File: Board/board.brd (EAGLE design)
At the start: 68.6 x 53.3 mm, 19 parts, among them IC1 L293D

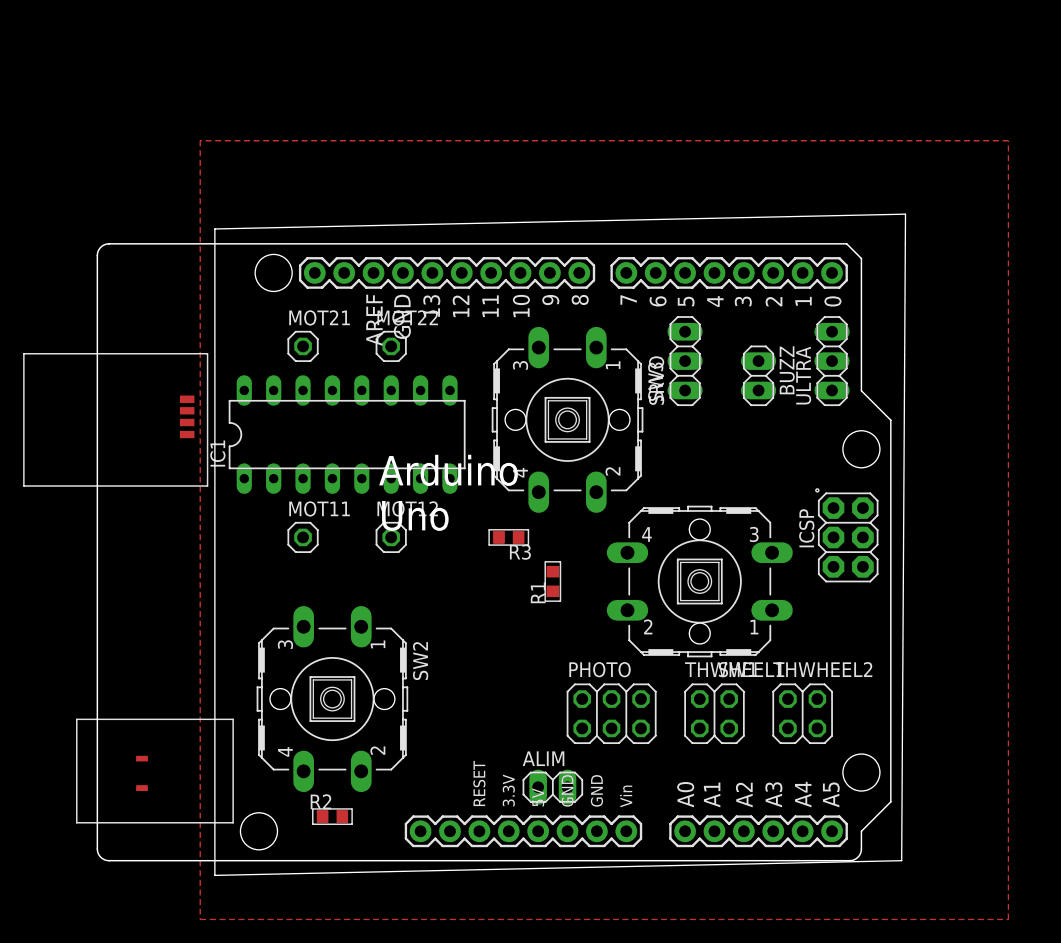
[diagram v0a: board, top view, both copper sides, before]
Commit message: Updated boad
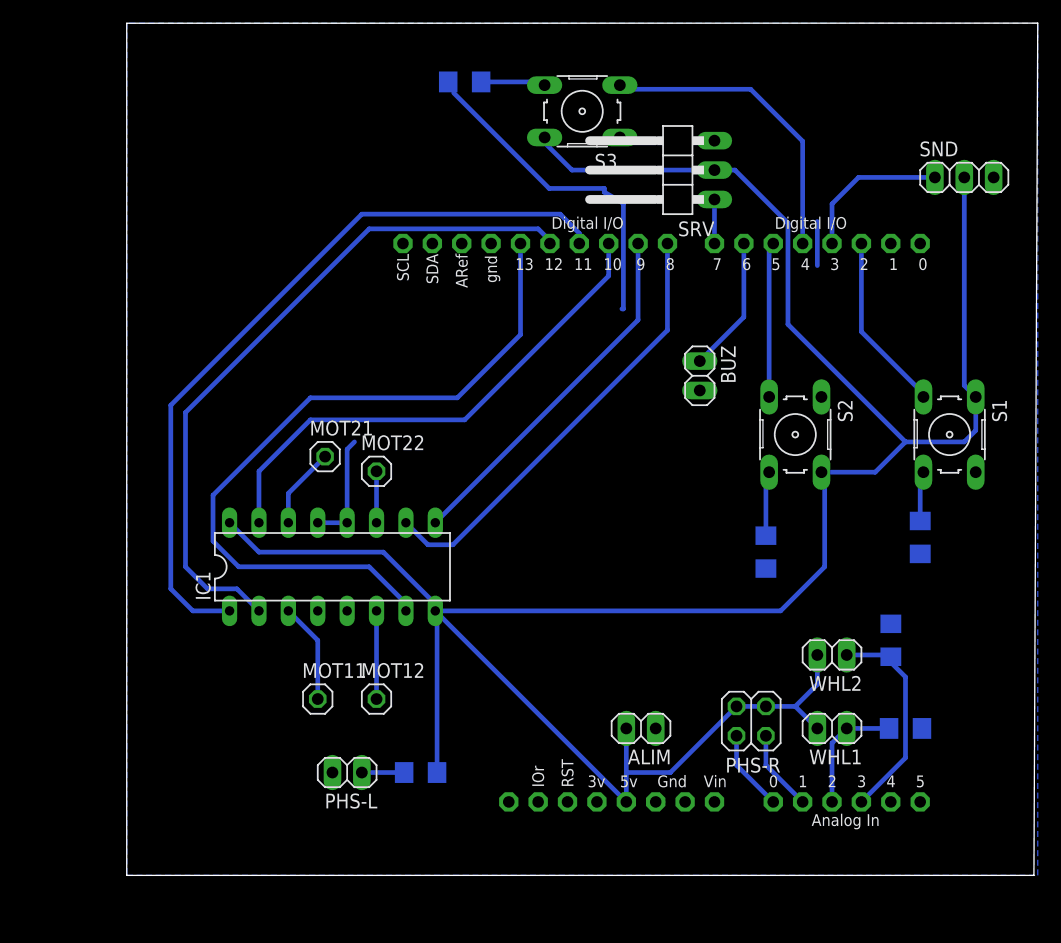
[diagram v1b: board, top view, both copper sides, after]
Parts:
- removed BUZZ: (no value), pinhead:1X02
- removed PCB1: ARDUINO_UNO, E14_Arduino_revB:ARDUINO_UNO
- removed PHOTO: (no value), pinhead:2X03
- removed SRVO, ULTRA: (no value), pinhead:1X03
- removed SW1, SW2, SW3: (no value), adafruit:B3F-40XX
- removed THWHEEL1, THWHEEL2: (no value), pinhead:2X02
- added BUZ, PHS-L, WHL1, WHL2: (no value), pinhead:1X02
- added PHS-R: (no value), pinhead:2X02
- added R4, R5: 10k, resistor:R1206
- added R6: 220, resistor:R1206
- added S1, S2, S3: (no value), switch-omron:B3F-10XX
- added SND: (no value), pinhead:1X03
- added SRV: (no value), pinhead:1X03/90
- added U1: ARDUINOR3-BPLACE, adafruit:ARDUINOR3-BPLACE
- ALIM: value (none) -> 5V
- R1, R2, R3: device BaseApp:R0603 -> resistor:R1206
- moved R2 43.9 mm to (65.4, 31.8), flipped to the bottom, turned to 90 degrees
- moved R3 39.6 mm to (39.4, 72.4), flipped to the bottom
- moved R1 32.0 mm to (78.7, 33.0), flipped to the bottom
- moved MOT11 14.0 mm to (26.7, 19.1)
- moved MOT12 14.0 mm to (31.8, 19.1)
- moved IC1 11.5 mm to (27.9, 30.5)
- moved MOT22 10.9 mm to (31.8, 38.7)
- moved MOT21 9.71 mm to (27.3, 40.0)
- moved ALIM 9.16 mm to (54.6, 16.5), turned to 180 degrees
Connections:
- removed net N$15: PCB1.3, ULTRA.2
- removed net N$17: PCB1.7, SW3.3
- new net 3V: U1.3V
- new net PIN12: IC1.2, U1.D12
- new net PIN13: IC1.7, U1.D13
- new net VIN: U1.VIN
- net +5V: now also PHS-R.1, PHS-R.3, R6.2, S1.1, S2.2, S3.2, SND.2, SRV.2, U1.5V, WHL1.2, WHL2.2; no longer PCB1.5V, PHOTO.1, PHOTO.3, PHOTO.5, SRVO.1, SW1.1, SW2.2, SW3.1, THWHEEL1.1, THWHEEL1.3, THWHEEL2.1, THWHEEL2.3, ULTRA.1
- net GND: now also BUZ.2, PHS-L.2, R4.1, R5.2, SND.3, SRV.3, U1.GND, U1.GND1, U1.GND2; no longer BUZZ.2, PCB1.GND., PCB1.GND.., PCB1.SCL, SRVO.3, THWHEEL1.2, THWHEEL2.2, ULTRA.3
- net N$10: now also U1.D11; no longer PCB1.11
- net N$11: now also R4.2, U1.A2, WHL1.1; no longer PCB1.A1, PHOTO.6
- net N$12: now also PHS-L.1, R6.1; no longer PCB1.A0, PHOTO.4
- net N$13: now also R5.1, U1.A3, WHL2.1; no longer PHOTO.2
- net N$14: now also SRV.1, U1.D7; no longer PCB1.6, SRVO.2
- net N$16: now also BUZ.1, U1.D6; no longer BUZZ.1, PCB1.5
- net N$18: now also R2.2, S2.4; no longer R3.2, SW3.4
- net N$19: now also S3.3, U1.D4; no longer PCB1.4, SW2.3
- net N$20: now also R3.2, S3.4; no longer R2.2, SW2.4
- net N$21: now also S1.4; no longer SW1.4
- net N$22: now also SND.1, U1.D3; no longer PCB1.A2, THWHEEL1.4
- net N$23: now also S2.3, U1.D5; no longer PCB1.A3, THWHEEL2.4
- net N$24: now also S1.3, U1.D2; no longer PCB1.2, SW1.3
- net N$5: now also PHS-R.2, U1.A1; no longer IC1.2, PCB1.12
- net N$6: now also PHS-R.4, U1.A0; no longer IC1.7, PCB1.13
- net N$7: now also U1.D10; no longer PCB1.10
- net N$8: now also U1.D9; no longer PCB1.9
- net N$9: now also U1.D8; no longer PCB1.8
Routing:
- net +5V: track 0.00 -> 218.0 mm
- net N$10: track 0.00 -> 65.5 mm
- net PIN13: track 0.00 -> 63.7 mm
- net PIN12: track 0.00 -> 60.0 mm
- net N$7: track 0.00 -> 44.5 mm
- net GND: track 0.00 -> 42.2 mm
- net N$9: track 0.00 -> 38.6 mm
- net N$8: track 0.00 -> 31.4 mm
- net N$19: track 0.00 -> 26.6 mm
- net N$13: track 0.00 -> 18.6 mm
- net N$24: track 0.00 -> 15.4 mm
- net N$23: track 0.00 -> 13.4 mm
- net N$22: track 0.00 -> 13.3 mm
- net N$16: track 0.00 -> 11.7 mm
- net N$11: track 0.00 -> 10.5 mm
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- added copper zone on layer 16, net GND
- removed copper zone on layer 1, net GND
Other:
- board size 68.6 x 53.3 mm -> 78.7 x 73.7 mm
